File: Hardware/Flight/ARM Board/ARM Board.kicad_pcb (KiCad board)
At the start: 2 copper layers, 80 x 80 mm, 49 parts, among them J1 USB_OTG, J2 Conn_01x10, J3 SD_WM6698CT-ND, J4 Conn_01x20_Female, J5 Harwin_M80-5400642, J6 SD_WM6698CT-ND, J7 1053131202, U2 STM32L4x6RxT6, U3 SRAM_23LC1024T-I_ST, U4 MCP2562, U5 FT230XS, Y1 Crystal_GND23

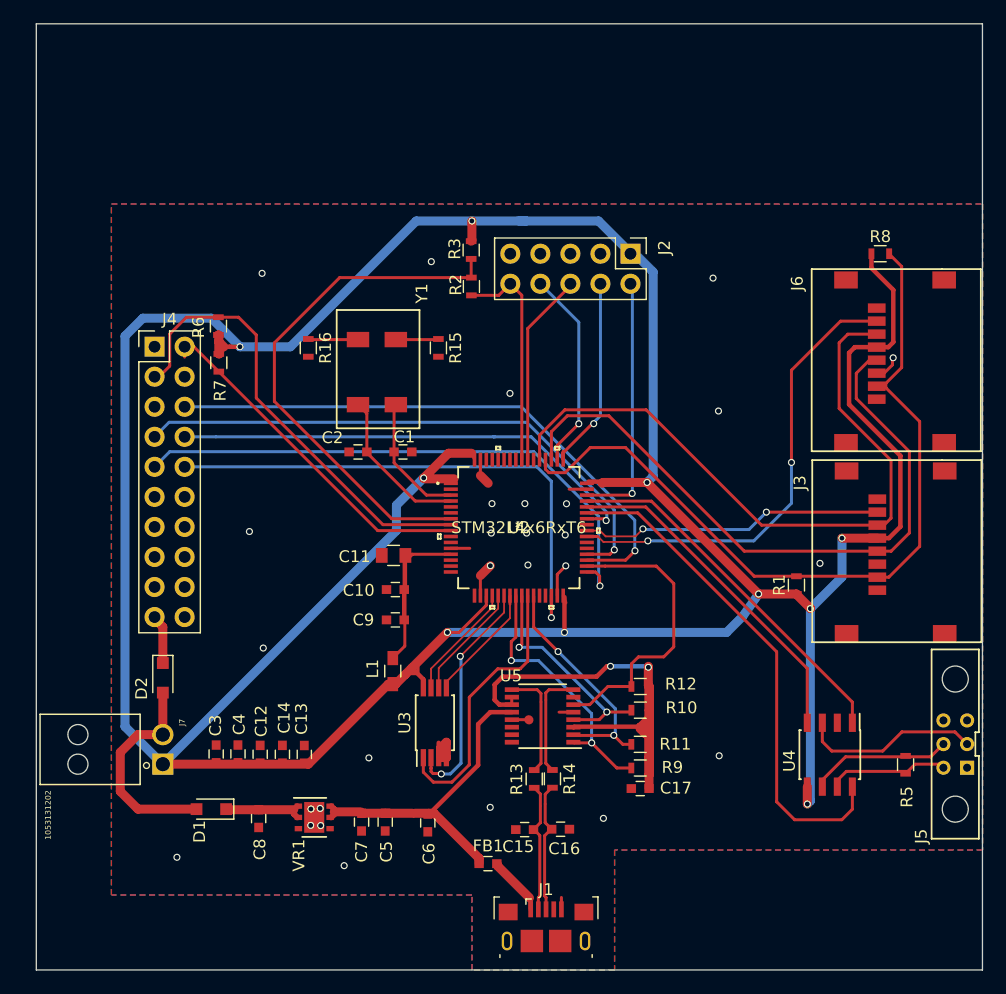
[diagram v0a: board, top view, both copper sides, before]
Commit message: starting rev2 of board layout
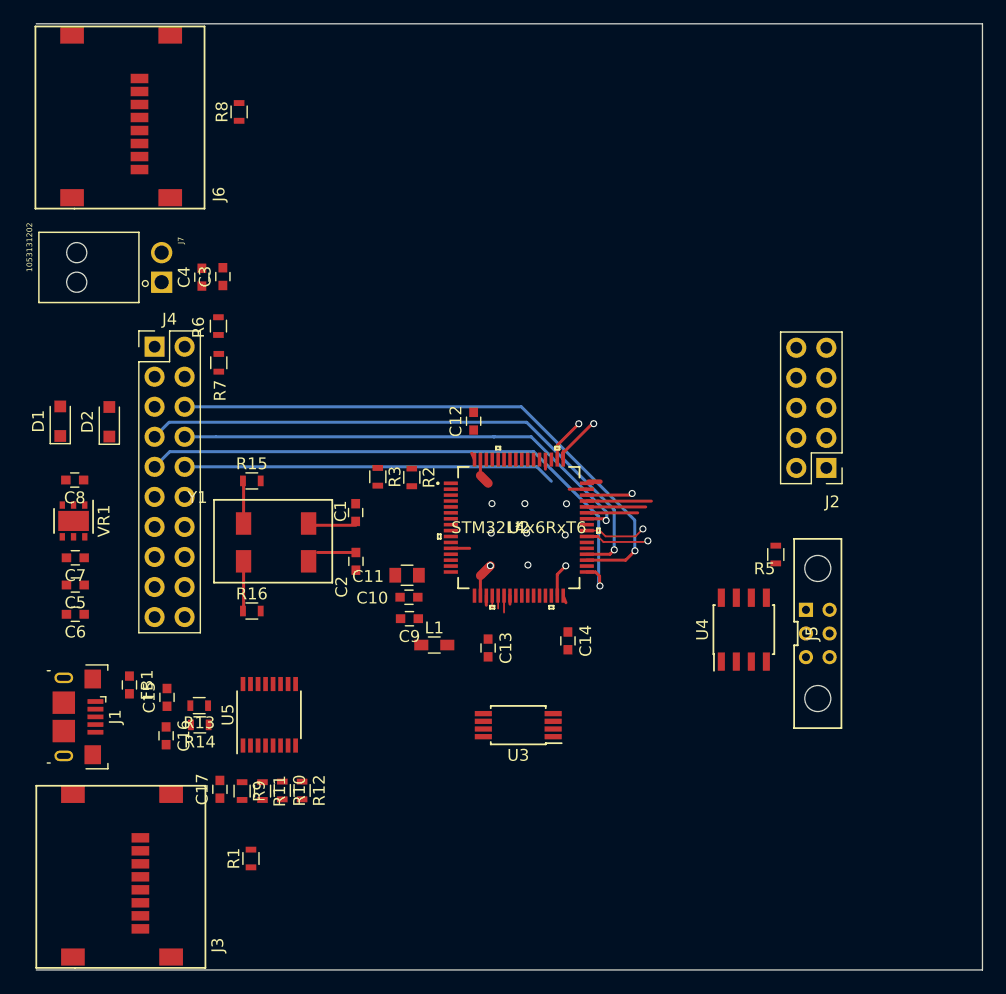
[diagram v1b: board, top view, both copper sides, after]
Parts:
- moved J3 72.1 mm to (8.80, 76.5), turned to 90 degrees
- moved J6 63.4 mm to (8.72, 12.3), turned to 90 degrees
- moved R8 55.5 mm to (17.1, 7.45), turned to 90 degrees
- moved R1 51.6 mm to (18.1, 70.6)
- moved J1 44.5 mm to (2.67, 58.6), turned to 270 degrees
- moved J7 40.8 mm to (10.6, 21.9)
- moved C4 40.4 mm to (14.0, 21.4)
- moved C3 40.4 mm to (15.8, 21.4)
- moved C17 35.5 mm to (15.5, 64.7), turned to 90 degrees
- moved D1 35.2 mm to (2.02, 33.6), turned to 90 degrees
- moved C6 34.6 mm to (3.30, 49.9), turned to 180 degrees
- moved C16 34.3 mm to (11.0, 60.2), turned to 270 degrees
- moved FB1 33.9 mm to (7.88, 55.9), turned to 270 degrees
- moved R9 33.7 mm to (17.4, 64.9), turned to 270 degrees
- moved C12 33.4 mm to (37.0, 33.6)
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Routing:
- net VDD33: track 308.0 -> 3.05 mm, vias 10 -> 0
- net MISO3: track 66.8 -> 0.81 mm
- net MOSI3: track 57.1 -> 0.00 mm
- net SCK3: track 56.1 -> 0.00 mm
- net Net-(R2-Pad2): track 44.5 -> 0.00 mm
- net VCCIO: track 43.7 -> 0.00 mm, vias 2 -> 0
- net SCL: track 39.8 -> 0.00 mm
- net ~CAN_EN: track 42.6 -> 4.02 mm
- net ~CS3: track 38.9 -> 5.26 mm, vias 2 -> 1
- net SDA: track 30.1 -> 0.00 mm
- net VBUS: track 28.6 -> 0.00 mm
- net CANTX: track 31.2 -> 5.45 mm
- net UART_~CTS: track 24.9 -> 0.00 mm
- net CANRX: track 28.9 -> 4.98 mm
- net ~CS1: track 23.5 -> 0.00 mm
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- removed copper zone on B.Cu, net GND
- removed copper zone on F.Cu, net GND
